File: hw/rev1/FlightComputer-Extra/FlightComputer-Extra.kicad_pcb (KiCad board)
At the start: 2 copper layers, 128 x 19.8 mm, 21 parts, among them J1 SJ-43617-SMT, J2 Conn_01x10, J3 Conn_01x10, J4 IPEX_IPX, J5 Conn_DEBUG, U1 Teseo-LIV3F

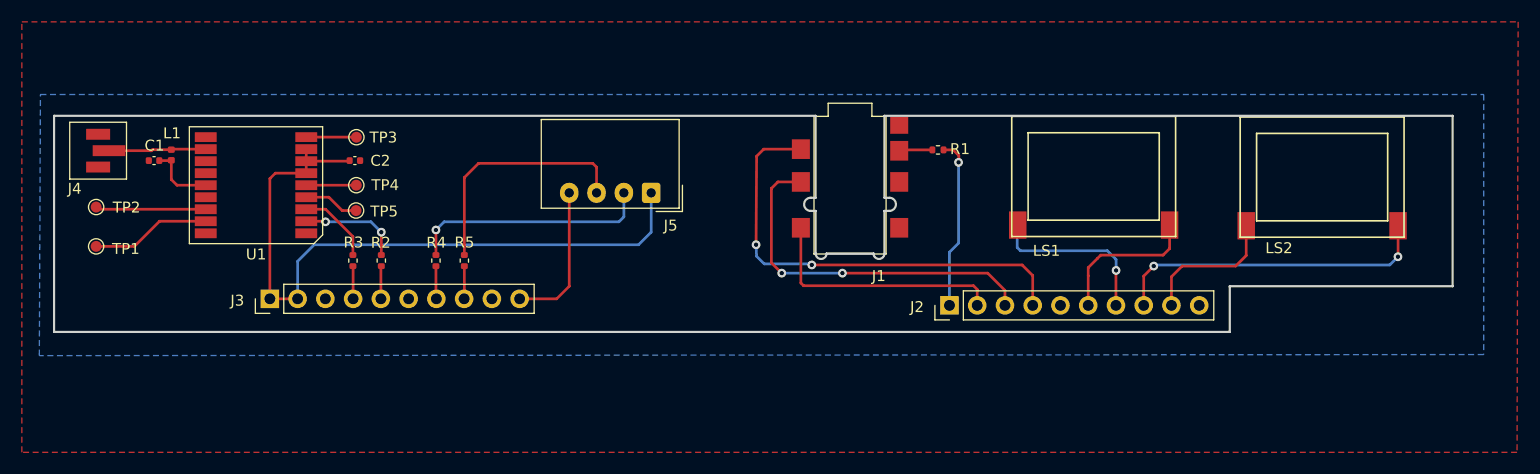
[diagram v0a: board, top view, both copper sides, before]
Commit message: ...
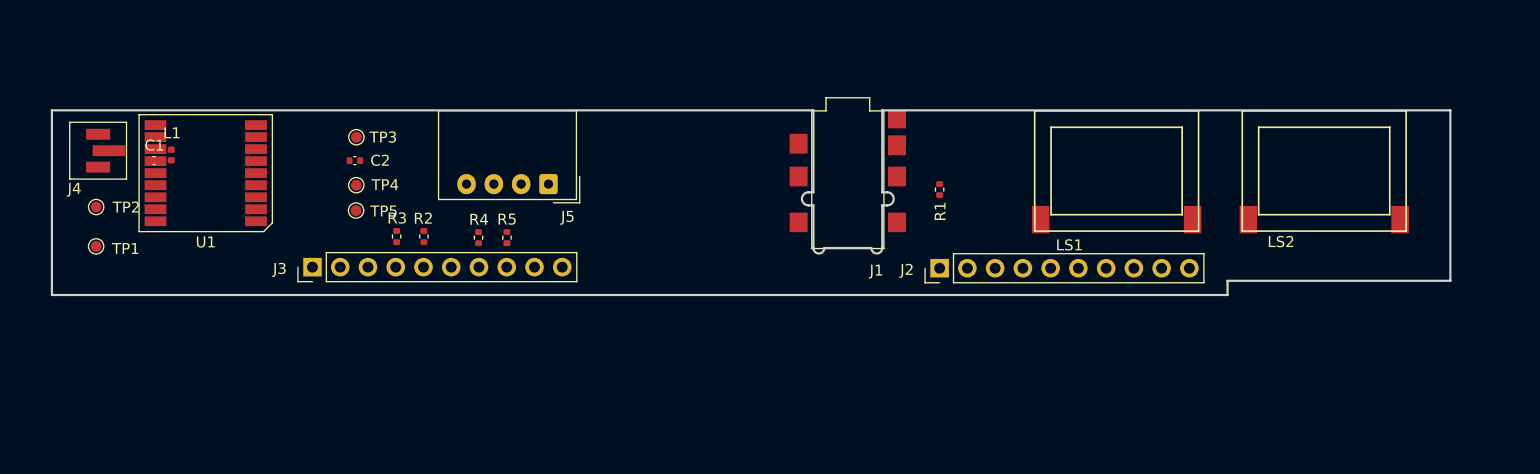
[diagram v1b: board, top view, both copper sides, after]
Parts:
- moved J5 9.43 mm to (121.4, 88.8)
- moved J3 4.86 mm to (99.8, 96.4)
- moved U1 4.73 mm to (90.0, 87.8)
- moved R3 4.57 mm to (107.5, 93.6)
- moved R2 4.48 mm to (110.0, 93.6)
- moved R4 4.43 mm to (115.0, 93.7)
- moved R5 4.43 mm to (117.6, 93.7)
- moved R1 3.63 mm to (157.2, 89.3), turned to 90 degrees
- moved J2 3.52 mm to (157.2, 96.5)
- moved LS1 2.16 mm to (173.4, 87.6)
- moved LS2 0.59 mm to (192.4, 87.6)
- moved J1 0.54 mm to (148.8, 82.1)
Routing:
- net VCC_PERIH: track 63.8 -> 0.00 mm
- net /HP_DETECT: track 42.2 -> 0.00 mm, vias 2 -> 0
- net /HP_RIGHT: track 33.5 -> 0.00 mm, vias 2 -> 0
- net /SPK_RP: track 29.5 -> 0.00 mm, vias 2 -> 0
- net /HP_LEFT: track 22.9 -> 0.00 mm
- net Net-(J5-Pad3): track 22.2 -> 0.00 mm
- net Net-(J5-Pad2): track 22.2 -> 0.00 mm, vias 1 -> 0
- net /SPK_LN: track 15.7 -> 0.00 mm, vias 1 -> 0
- net VCC_3V3: track 15.7 -> 0.00 mm, vias 1 -> 0
- net /SPK_LP: track 13.8 -> 0.00 mm
- net GND: track 13.6 -> 0.00 mm
- net /SPK_RN: track 13.0 -> 0.00 mm
- net Net-(TP1-Pad1): track 11.0 -> 0.00 mm
- net Net-(TP2-Pad1): track 10.1 -> 0.00 mm
- net Net-(R2-Pad2): track 9.37 -> 0.00 mm, vias 2 -> 0
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- removed copper zone on B.Cu, net GND
- removed copper zone on F.Cu, net GND
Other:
- board size 128 x 19.8 mm -> 128 x 16.9 mm
